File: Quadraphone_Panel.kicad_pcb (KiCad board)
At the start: 2 copper layers, 60.8 x 128.5 mm, 31 parts

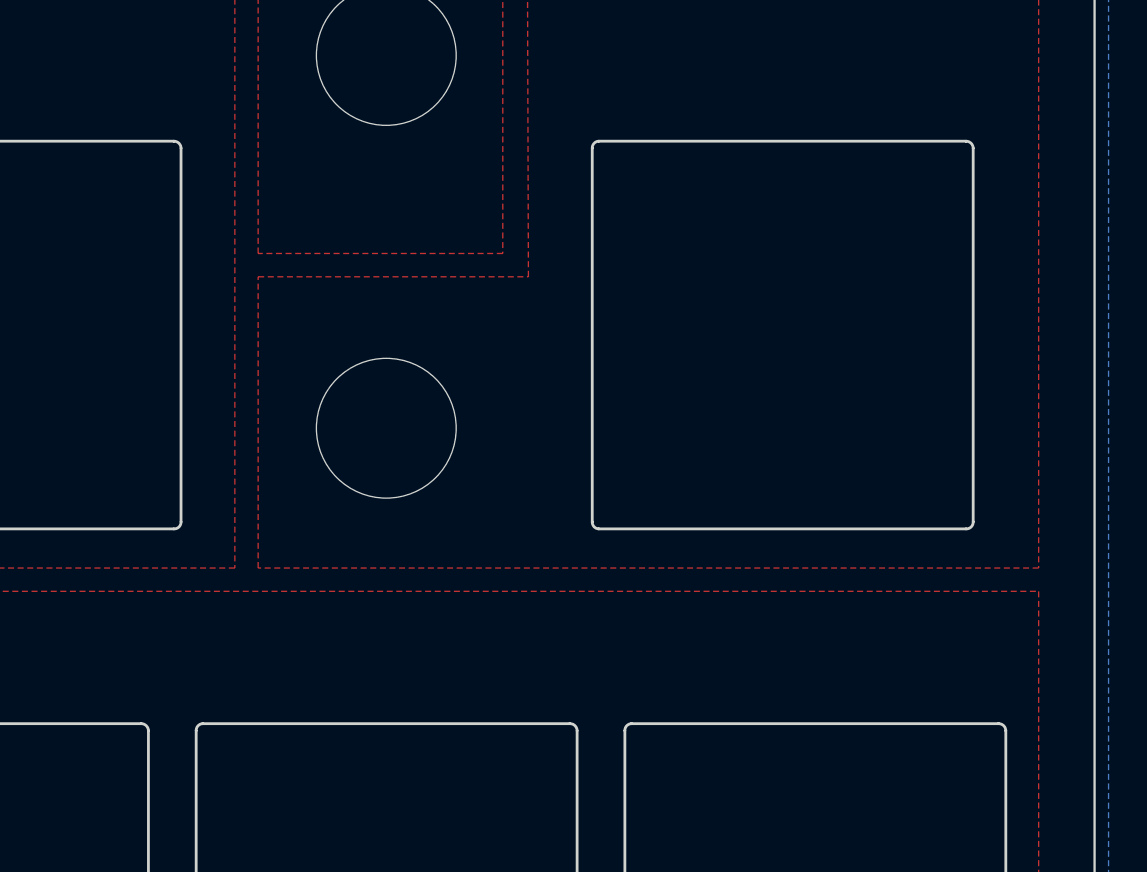
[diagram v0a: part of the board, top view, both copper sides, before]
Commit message: Prepared all gerbers
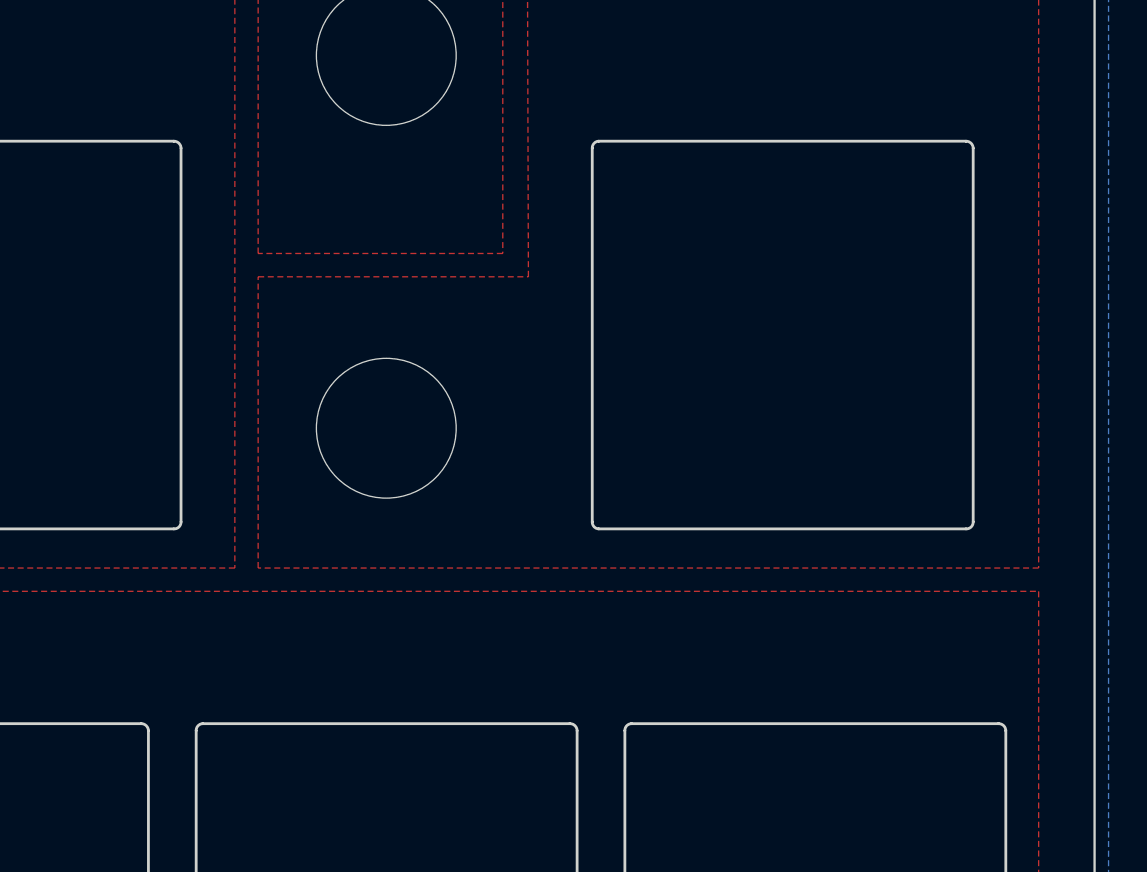
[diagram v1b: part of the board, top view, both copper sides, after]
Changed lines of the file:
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@@
     (0 "F.Cu" signal)
     (31 "B.Cu" signal)
-    (32 "B.Adhes" user "B.Adhesive")
-    (33 "F.Adhes" user "F.Adhesive")
     (34 "B.Paste" user)
     (35 "F.Paste" user)
@@
     (40 "Dwgs.User" user "User.Drawings")
     (41 "Cmts.User" user "User.Comments")
-    (42 "Eco1.User" user "User.Eco1")
-    (43 "Eco2.User" user "User.Eco2")
     (44 "Edge.Cuts" user)
     (45 "Margin" user)
@@
     (48 "B.Fab" user)
     (49 "F.Fab" user)
-    (50 "User.1" user)
-    (51 "User.2" user)
-    (52 "User.3" user)
-    (53 "User.4" user)
-    (54 "User.5" user)
-    (55 "User.6" user)
-    (56 "User.7" user)
-    (57 "User.8" user)
-    (58 "User.9" user)
   )
   (setup
@@
       (outputformat 1)
       (mirror false)
-      (drillshape 1)
+      (drillshape 0)
       (scaleselection 1)
-      (outputdirectory "")
+      (outputdirectory "Gerbers/Panel/")
     )
   )
@@
     (attr board_only exclude_from_pos_files exclude_from_bom)
     (fp_text reference "kibuzzard-63D25E01" (at 0 -4.869077) (layer "F.SilkS") hide
-      (effects (font (size 0 0)))
+      (effects (font (size 0 0) (thickness 0.15)))
     )
     (fp_text value "G***" (at 0 4.869077) (layer "F.SilkS") hide
-      (effects (font (size 0 0)))
+      (effects (font (size 0 0) (thickness 0.15)))
     )
     (fp_poly (pts
@@
     (fp_line (start -8.16 -8.02) (end -8.16 8.02) (layer "Edge.Cuts") (width 0.12))
     (fp_arc (start 8.19 8.02) (mid 8.100917 8.238111) (end 7.88 8.32) (layer "Edge.Cuts") (width 0.12))
-    (fp_arc (start 7.88 -8.32) (mid 8.096622 -8.233665) (end 8.19 -8.02) (layer "Edge.Cuts") (width 0.12))
+    (fp_arc (start 7.88 -8.32) (mid 8.096588 -8.233658) (end 8.19 -8.02) (layer "Edge.Cuts") (width 0.12))
     (fp_arc (start -7.88 8.32) (mid -8.081749 8.227632) (end -8.16 8.02) (layer "Edge.Cuts") (width 0.12))
     (fp_arc (start -8.16 -8.02) (mid -8.081443 -8.227347) (end -7.88 -8.32) (layer "Edge.Cuts") (width 0.12))
@@
     (fp_arc (start -8.16 -8.02) (mid -8.081443 -8.227347) (end -7.88 -8.32) (layer "Edge.Cuts") (width 0.12))
     (fp_arc (start 8.19 8.02) (mid 8.100917 8.238111) (end 7.88 8.32) (layer "Edge.Cuts") (width 0.12))
-    (fp_arc (start 7.88 -8.32) (mid 8.096622 -8.233665) (end 8.19 -8.02) (layer "Edge.Cuts") (width 0.12))
+    (fp_arc (start 7.88 -8.32) (mid 8.096588 -8.233658) (end 8.19 -8.02) (layer "Edge.Cuts") (width 0.12))
     (fp_line (start -8.31 -8.5) (end -8.31 8.5) (layer "F.CrtYd") (width 0.05))
     (fp_line (start 8.39 -8.5) (end 8.39 8.5) (layer "F.CrtYd") (width 0.05))
@@
     (attr board_only exclude_from_pos_files exclude_from_bom)
     (fp_text reference "kibuzzard-63D2A377" (at 0 -4.760221) (layer "F.SilkS") hide
-      (effects (font (size 0 0)))
+      (effects (font (size 0 0) (thickness 0.15)))
     )
     (fp_text value "G***" (at 0 4.760221) (layer "F.SilkS") hide
-      (effects (font (size 0 0)))
+      (effects (font (size 0 0) (thickness 0.15)))
     )
     (fp_poly (pts
@@
     (attr board_only exclude_from_pos_files exclude_from_bom)
     (fp_text reference "kibuzzard-63D2A3C5" (at 0 -4.68697) (layer "F.SilkS") hide
-      (effects (font (size 0 0)))
+      (effects (font (size 0 0) (thickness 0.15)))
     )
     (fp_text value "G***" (at 0 4.68697) (layer "F.SilkS") hide
-      (effects (font (size 0 0)))
+      (effects (font (size 0 0) (thickness 0.15)))
     )
     (fp_poly (pts
@@
     (attr board_only exclude_from_pos_files exclude_from_bom)
     (fp_text reference "kibuzzard-63D25EC7" (at 0 -4.728828 90) (layer "F.SilkS") hide
-      (effects (font (size 0 0)))
+      (effects (font (size 0 0) (thickness 0.15)))
     )
     (fp_text value "G***" (at 0 4.728828 90) (layer "F.SilkS") hide
-      (effects (font (size 0 0)))
+      (effects (font (size 0 0) (thickness 0.15)))
     )
     (fp_poly (pts
@@
     (fp_arc (start -8.16 -8.02) (mid -8.081443 -8.227347) (end -7.88 -8.32) (layer "Edge.Cuts") (width 0.12))
     (fp_arc (start 8.19 8.02) (mid 8.100917 8.238111) (end 7.88 8.32) (layer "Edge.Cuts") (width 0.12))
-    (fp_arc (start 7.88 -8.32) (mid 8.096622 -8.233665) (end 8.19 -8.02) (layer "Edge.Cuts") (width 0.12))
+    (fp_arc (start 7.88 -8.32) (mid 8.096588 -8.233658) (end 8.19 -8.02) (layer "Edge.Cuts") (width 0.12))
     (fp_line (start 8.39 -8.5) (end 8.39 8.5) (layer "F.CrtYd") (width 0.05))
     (fp_line (start -8.31 -8.5) (end -8.31 8.5) (layer "F.CrtYd") (width 0.05))
@@
     (fp_line (start 7.88 -8.32) (end -7.88 -8.32) (layer "Edge.Cuts") (width 0.12))
     (fp_arc (start -7.88 8.32) (mid -8.081749 8.227632) (end -8.16 8.02) (layer "Edge.Cuts") (width 0.12))
-    (fp_arc (start 7.88 -8.32) (mid 8.096622 -8.233665) (end 8.19 -8.02) (layer "Edge.Cuts") (width 0.12))
+    (fp_arc (start 7.88 -8.32) (mid 8.096588 -8.233658) (end 8.19 -8.02) (layer "Edge.Cuts") (width 0.12))
     (fp_arc (start -8.16 -8.02) (mid -8.081443 -8.227347) (end -7.88 -8.32) (layer "Edge.Cuts") (width 0.12))
     (fp_arc (start 8.19 8.02) (mid 8.100917 8.238111) (end 7.88 8.32) (layer "Edge.Cuts") (width 0.12))
@@
     (fp_line (start -8.16 -8.02) (end -8.16 8.02) (layer "Edge.Cuts") (width 0.12))
     (fp_arc (start -7.88 8.32) (mid -8.081749 8.227632) (end -8.16 8.02) (layer "Edge.Cuts") (width 0.12))
-    (fp_arc (start 7.88 -8.32) (mid 8.096622 -8.233665) (end 8.19 -8.02) (layer "Edge.Cuts") (width 0.12))
+    (fp_arc (start 7.88 -8.32) (mid 8.096588 -8.233658) (end 8.19 -8.02) (layer "Edge.Cuts") (width 0.12))
     (fp_arc (start 8.19 8.02) (mid 8.100917 8.238111) (end 7.88 8.32) (layer "Edge.Cuts") (width 0.12))
     (fp_arc (start -8.16 -8.02) (mid -8.081443 -8.227347) (end -7.88 -8.32) (layer "Edge.Cuts") (width 0.12))
